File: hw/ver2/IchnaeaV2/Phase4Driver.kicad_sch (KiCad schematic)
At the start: 21 parts, among them Q14 MCAC80N10Y, Q15 MCAC80N10Y, Q16 MCAC80N10Y, Q17 MCAC80N10Y, U5 HIP2210

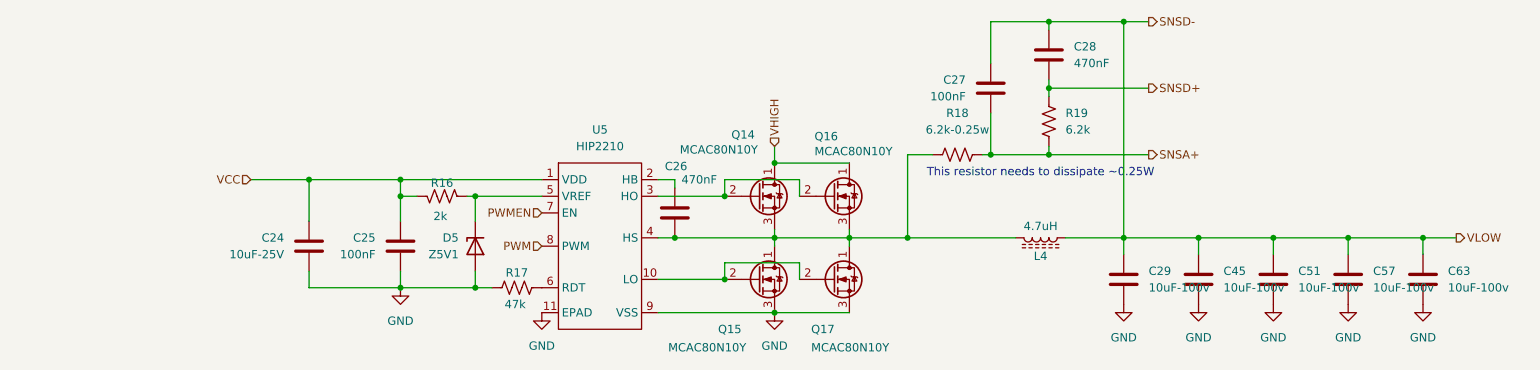
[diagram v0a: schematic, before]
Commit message: Sync work to main PC
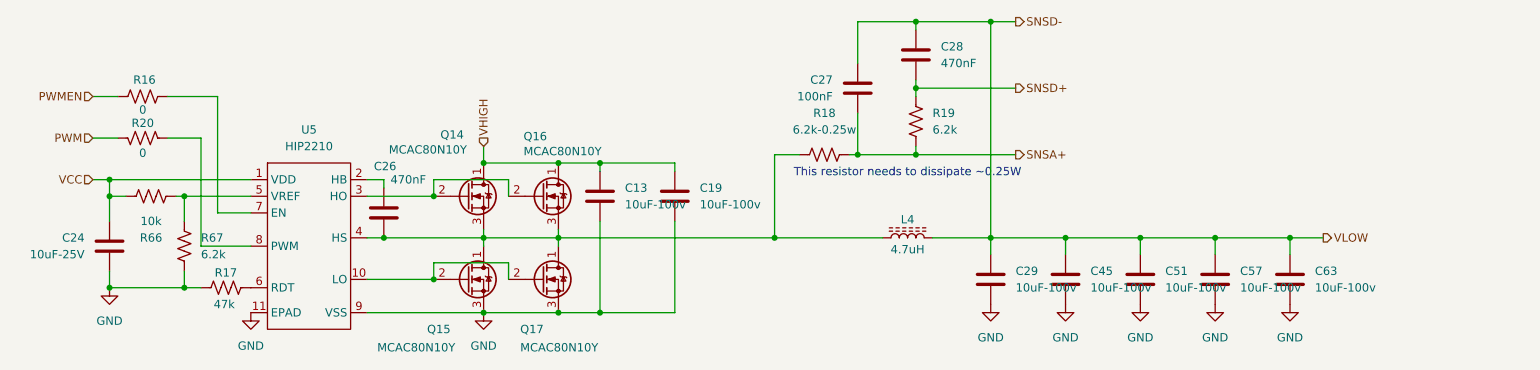
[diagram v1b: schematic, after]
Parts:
- removed C25: 100nF, Capacitor_SMD:C_0603_1608Metric, symbol Device:C
- removed D5: Z5V1, Diode_SMD:D_SOD-123, symbol Device:D_Zener
- added C13, C19: 10uF-100v, Capacitor_SMD:C_1210_3225Metric_Pad1.33x2.70mm_HandSolder, symbol Device:C
- added R20: 0, Resistor_SMD:R_0603_1608Metric, symbol Device:R_US
- added R66: 10k, Resistor_SMD:R_0603_1608Metric, symbol Device:R_US
- added R67: 6.2k, Resistor_SMD:R_0603_1608Metric, symbol Device:R_US
- R16: value 2k -> 0; LCSC (none) -> C21189
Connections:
- net GND: now also C13.2, C19.2, R67.2
- net PWM: now also R20.2; no longer U5.8 (PWM)
- net PWMEN: now also R16.2; no longer U5.7 (EN)
- net SNSD-: now also L4.2; no longer L4.1
- net VCC: now also R66.1; no longer R16.2
- net VHIGH: now also C13.1, C19.1
- net at C26.2, Q14.3 (S), Q15.1 (D)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: now also L4.1; no longer L4.2
- net at R16.1: now also U5.7 (EN); no longer U5.5 (VREF)
- new net: R20.1, U5.8 (PWM)
- new net: R66.2, R67.1, U5.5 (VREF)
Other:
- moved on the sheet: C24, C26, C27, C28, C29, C45, C51, C57, C63, L4, Q14, Q15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
